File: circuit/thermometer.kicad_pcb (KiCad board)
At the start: 2 copper layers, 137.2 x 77.5 mm, 43 parts, among them IC1 ICL7107CPL, IC2 4001, IC3 LM285Z-1.2, IC4 TMP36

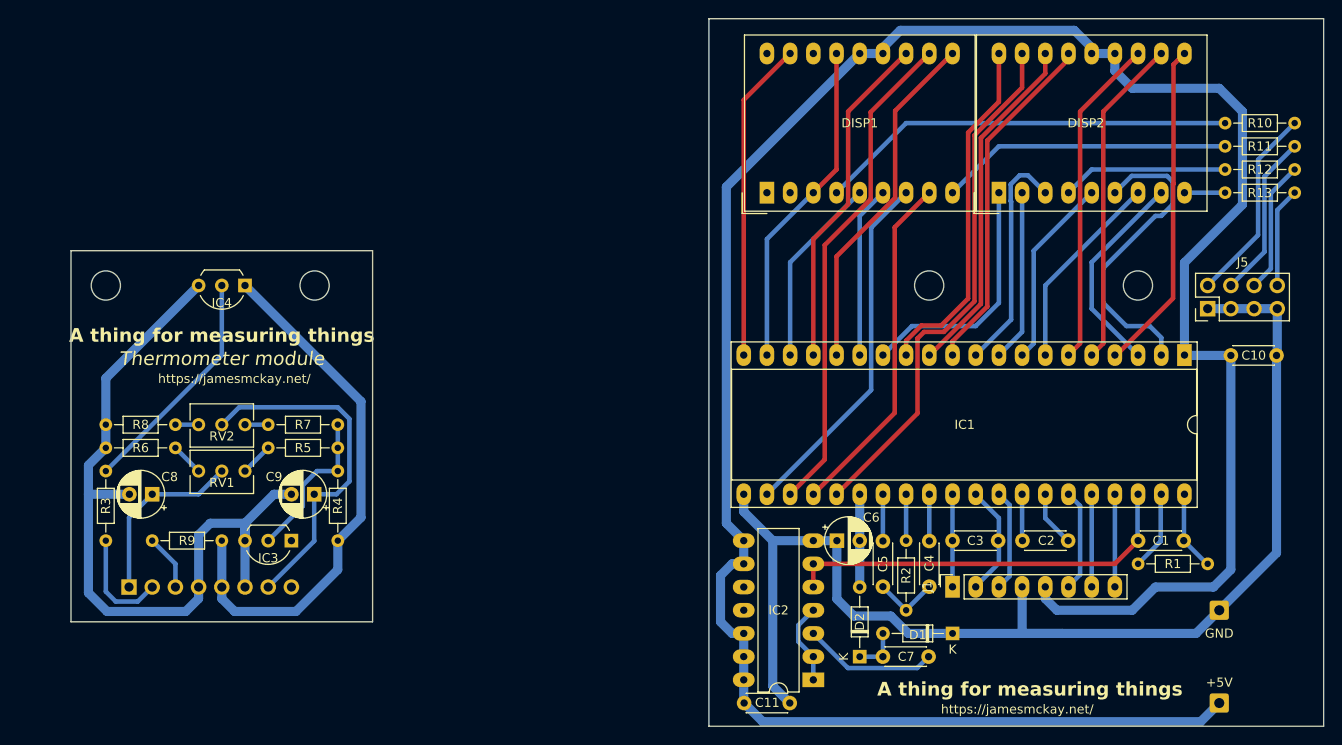
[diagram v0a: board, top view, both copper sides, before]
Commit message: A bit more tidying up
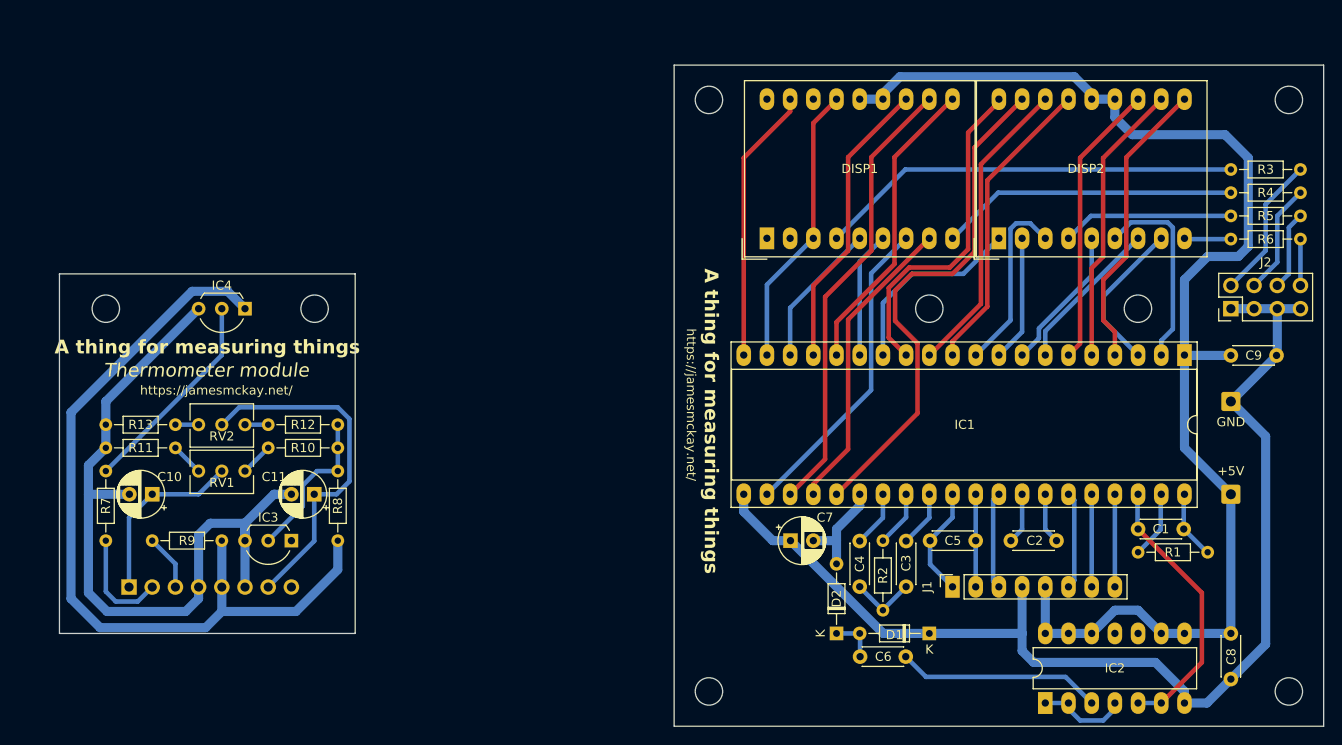
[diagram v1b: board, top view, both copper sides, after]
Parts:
- removed the C3 at (165.0, 78.7)
- removed the REF** at (67.3, 50.8)
- removed the REF** at (90.2, 50.8)
- removed the REF** at (180.3, 50.8)
- removed the REF** at (157.5, 50.8)
- added C5: 10nF, Capacitor_THT:C_Disc_D4.3mm_W1.9mm_P5.00mm, F.Cu at (157.6, 78.7)
- added REF**: MountingHole_3mm, MountingHole:MountingHole_3mm, F.Cu at (133.3, 95.2)
- added REF**: MountingHole_3mm, MountingHole:MountingHole_3mm, F.Cu at (196.8, 95.2)
- added REF**: MountingHole_3mm, MountingHole:MountingHole_3mm, F.Cu at (180.3, 53.3)
- added REF**: MountingHole_3mm, MountingHole:MountingHole_3mm, F.Cu at (157.5, 53.3)
- added REF**: MountingHole_3mm, MountingHole:MountingHole_3mm, F.Cu at (196.8, 30.5)
- added REF**: MountingHole_3mm, MountingHole:MountingHole_3mm, F.Cu at (67.3, 53.3)
- added REF**: MountingHole_3mm, MountingHole:MountingHole_3mm, F.Cu at (90.2, 53.3)
- added REF**: MountingHole_3mm, MountingHole:MountingHole_3mm, F.Cu at (133.3, 30.5)
- moved C8 53.8 mm to (190.5, 88.9), turned to -90 degrees
- moved IC2 25.5 mm to (170.2, 96.5), turned to 90 degrees
- moved J3 22.9 mm to (190.5, 73.7)
- moved J4 22.9 mm to (190.5, 63.5)
- moved R3 5.12 mm to (198.1, 38.1)
- moved R4 5.12 mm to (190.5, 40.6)
- moved R5 5.12 mm to (190.5, 43.2)
- moved R6 5.12 mm to (190.5, 45.7)
- moved C7 5.08 mm to (142.3, 78.7)
- moved DISP1 5.00 mm to (139.7, 45.6)
- moved DISP2 5.00 mm to (165.1, 45.6)
- moved D2 3.60 mm to (147.3, 88.9)
- moved D1 2.55 mm to (157.5, 88.9)
- moved IC4 2.54 mm to (82.5, 53.3)
- moved C3 2.54 mm to (154.9, 83.8)
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- renumbered C8 to C10, C9 to C11, C4 to C3, C5 to C4, C7 to C6, C6 to C7, C11 to C8, C10 to C9, J5 to J2, +5V to J3, GND to J4, J2 to J5, R5 to R10, R6 to R11, R7 to R12, R8 to R13, R10 to R3, R11 to R4, R12 to R5, R13 to R6, R3 to R7, R4 to R8
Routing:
- net +5V: track 264.2 -> 139.5 mm
- net Net-(IC4-+V_{S}): track 59.0 -> 89.8 mm
- net Net-(IC1-OSC3): track 44.2 -> 30.1 mm
- net Net-(DISP2-d2): track 34.0 -> 21.8 mm
- net GND: track 135.6 -> 125.3 mm
- net Net-(C6-Pad2): track 14.7 -> 22.5 mm
- net Net-(DISP1-b1): track 36.2 -> 29.9 mm
- net Net-(DISP2-c2): track 23.0 -> 17.0 mm
- net Net-(J2-Pin_6): track 14.5 -> 8.67 mm
- net Net-(J2-Pin_8): track 10.9 -> 5.08 mm
- net Net-(J2-Pin_4): track 18.1 -> 12.3 mm
- net Net-(J2-Pin_2): track 21.7 -> 15.9 mm
- net Net-(DISP2-e1): track 27.1 -> 21.3 mm
- net Net-(DISP2-c1): track 25.3 -> 20.1 mm
- net Net-(DISP2-f2): track 36.2 -> 31.1 mm
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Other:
- board size 137.2 x 77.5 mm -> 138.4 x 72.4 mm
